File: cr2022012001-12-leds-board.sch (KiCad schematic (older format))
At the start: 38 parts, among them J1 USB_B_Micro, J2 Conn_01x04, SW1 SW_Push, U1 ATtiny85-20PU

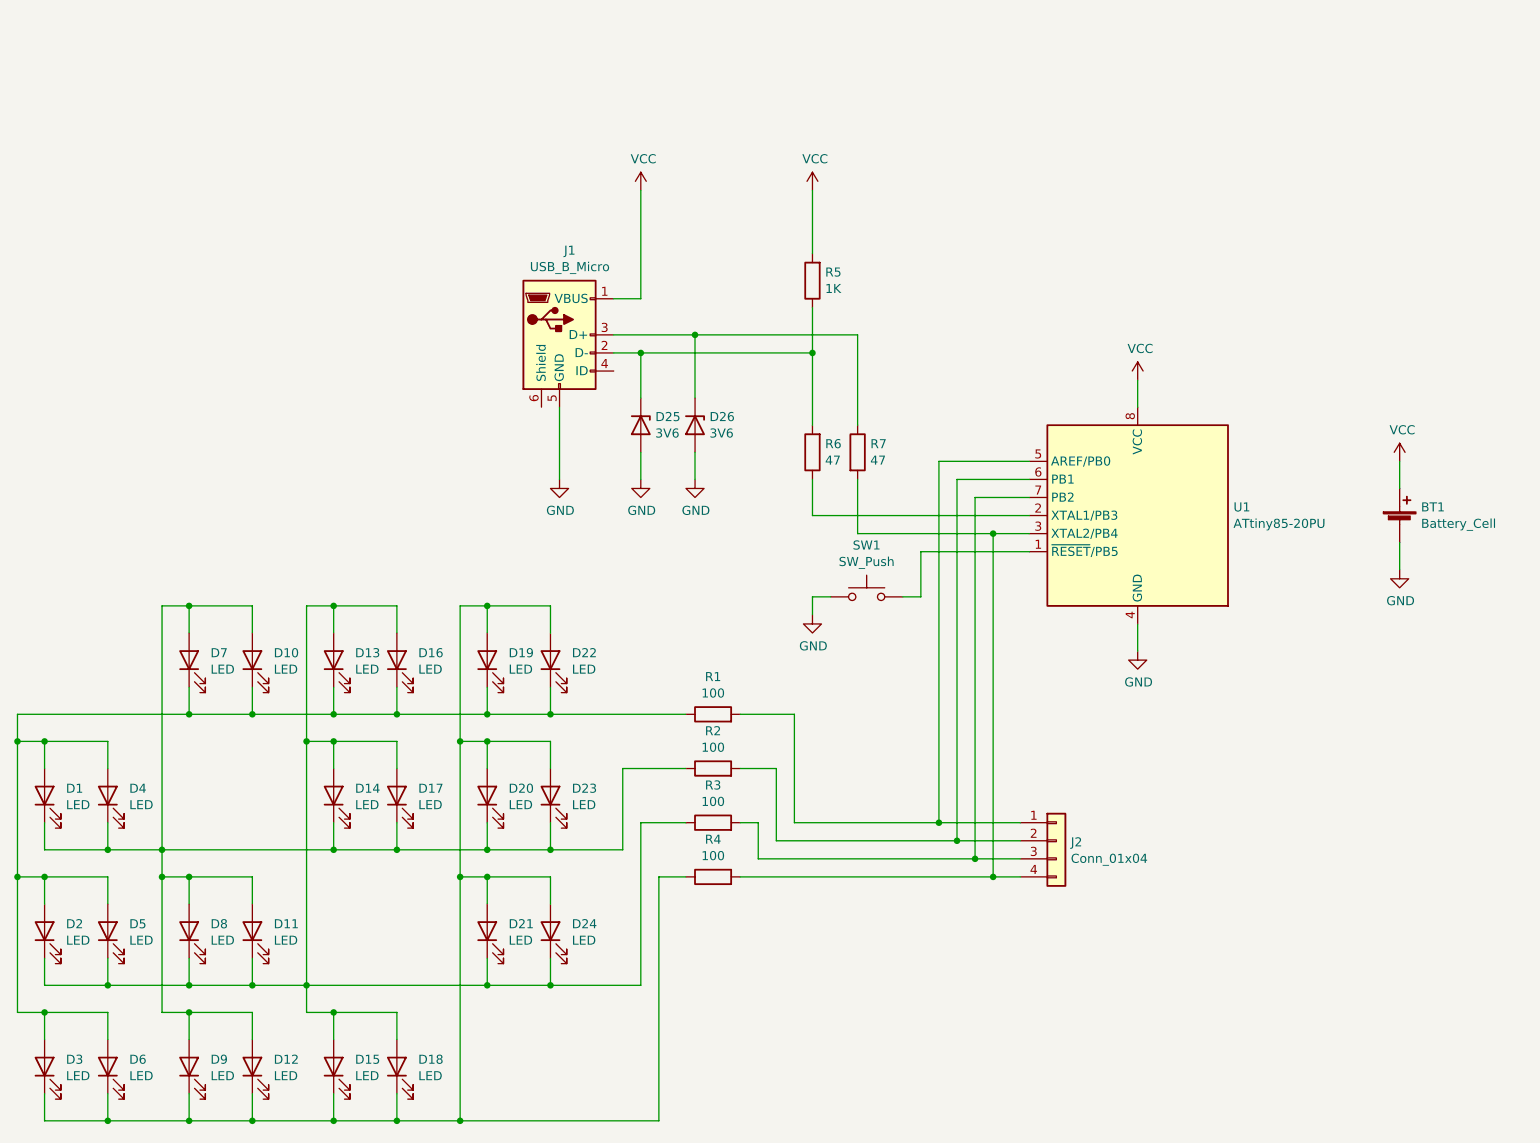
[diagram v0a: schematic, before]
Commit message: updated drawing
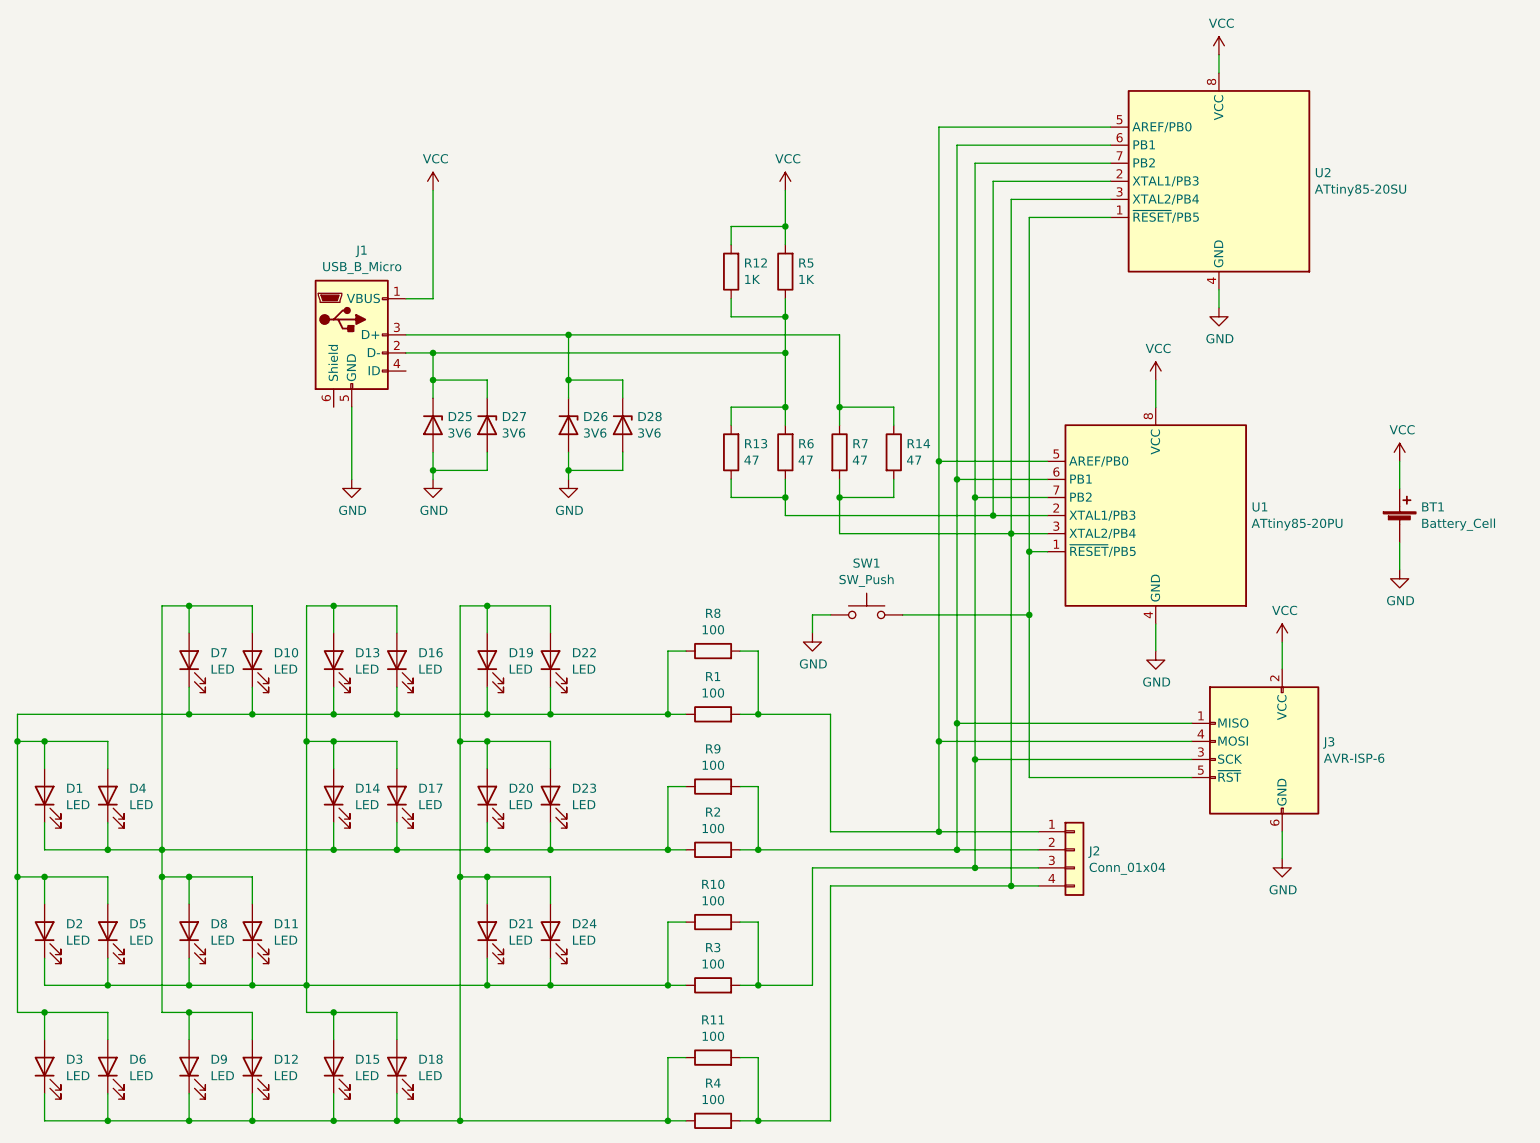
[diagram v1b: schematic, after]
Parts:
- added D27, D28: 3V6, Diode_THT:D_DO-41_SOD81_P7.62mm_Horizontal, symbol Device:D_Zener
- added J3: AVR-ISP-6, Connector_PinSocket_2.54mm:PinSocket_2x03_P2.54mm_Vertical, symbol Connector:AVR-ISP-6
- added R10, R11, R8, R9: 100, Resistor_SMD:R_0603_1608Metric_Pad0.98x0.95mm_HandSolder, symbol Device:R
- added R12: 1K, Resistor_SMD:R_0603_1608Metric_Pad0.98x0.95mm_HandSolder, symbol Device:R
- added R13, R14: 47, Resistor_SMD:R_0603_1608Metric_Pad0.98x0.95mm_HandSolder, symbol Device:R
- added U2: ATtiny85-20SU, Package_SO:SOIJ-8_5.3x5.3mm_P1.27mm, symbol MCU_Microchip_ATtiny:ATtiny85-20SU
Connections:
- net GND: now also D27.2 (A), D28.2 (A), J3.6 (GND), U2.4 (GND)
- net VCC: now also J3.2 (VCC), R12.2, U2.8 (VCC)
- net at D1.2 (A), D10.1 (K), D13.1 (K)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: now also R8.1
- net at J2.1 (Pin_1), R1.2, U1.5 (AREF/PB0): now also J3.4 (MOSI), R8.2, U2.5 (AREF/PB0)
- net at D1.1 (K), D10.2 (A), D11.2 (A)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: now also R9.1
- net at J2.2 (Pin_2), R2.2, U1.6 (PB1): now also J3.1 (MISO), R9.2, U2.6 (PB1)
- net at D11.1 (K), D13.2 (A), D14.2 (A)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: now also R10.1
- net at D12.1 (K), D15.1 (K), D18.1 (K)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: now also R11.1
- net at J2.3 (Pin_3), R3.2, U1.7 (PB2): now also J3.3 (SCK), R10.2, U2.7 (PB2)
- net at J2.4 (Pin_4), R4.2, R7.2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: now also R11.2, R14.2, U2.3 (XTAL2/PB4)
- net at D25.1 (K), J1.2 (D-), R5.1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: now also D27.1 (K), R12.1, R13.2
- net at D26.1 (K), J1.3 (D+), R7.1: now also D28.1 (K), R14.1
- net at SW1.2, U1.1 (~RESET~/PB5): now also J3.5 (~RST), U2.1 (~RESET~/PB5)
- net at R6.1, U1.2 (XTAL1/PB3): now also R13.1, U2.2 (XTAL1/PB3)
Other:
- moved on the sheet: D25, D26, J1, J2, R2, R3, R4, R5, R6, R7, SW1, U1

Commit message: revNC
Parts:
- J1: footprint Connector_USB:USB_Micro-B_Molex-105017-0001 -> Connector_USB:USB_Micro-B_Amphenol_10118194_Horizontal
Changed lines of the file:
@@
 F 0 "J1" H 3107 2767 50  0000 C CNN
 F 1 "USB_B_Micro" H 3107 2676 50  0000 C CNN
-F 2 "Connector_USB:USB_Micro-B_Molex-105017-0001" H 3200 2250 50  0001 C CNN
+F 2 "Connector_USB:USB_Micro-B_Amphenol_10118194_Horizontal" H 3200 2250 50  0001 C CNN
 F 3 "~" H 3200 2250 50  0001 C CNN
 	1    3050 2300
